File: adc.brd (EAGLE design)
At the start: 87.6 x 89.9 mm, 77 parts, among them IC13 4051D, IC5 4051D, IC6 4051D, U1 ADV7173KSTZ, U2 AD5308ARUZ, U3 AD7927BRUZ, U4 ADV7173KSTZ, U5 AD5308ARUZ, U6 AD5308ARUZ, U7 AD5308ARUZ

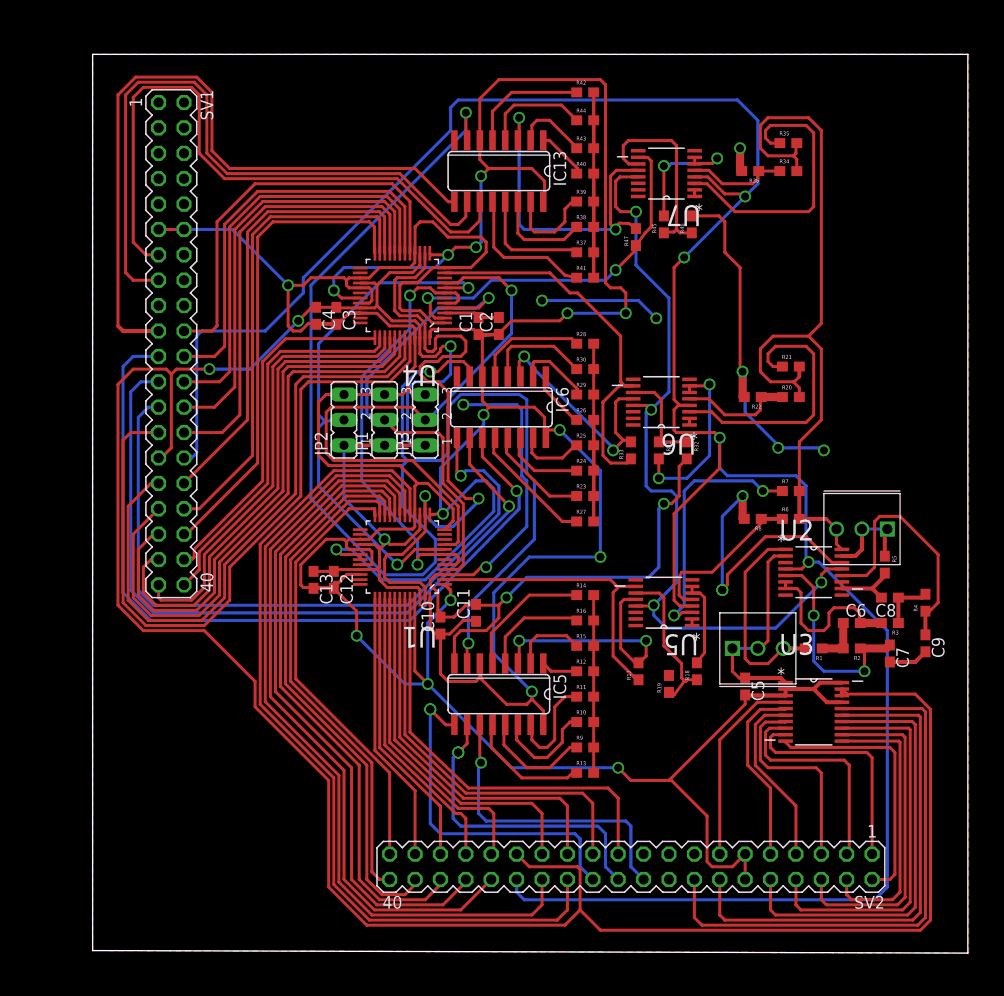
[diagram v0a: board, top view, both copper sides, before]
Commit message: autalização
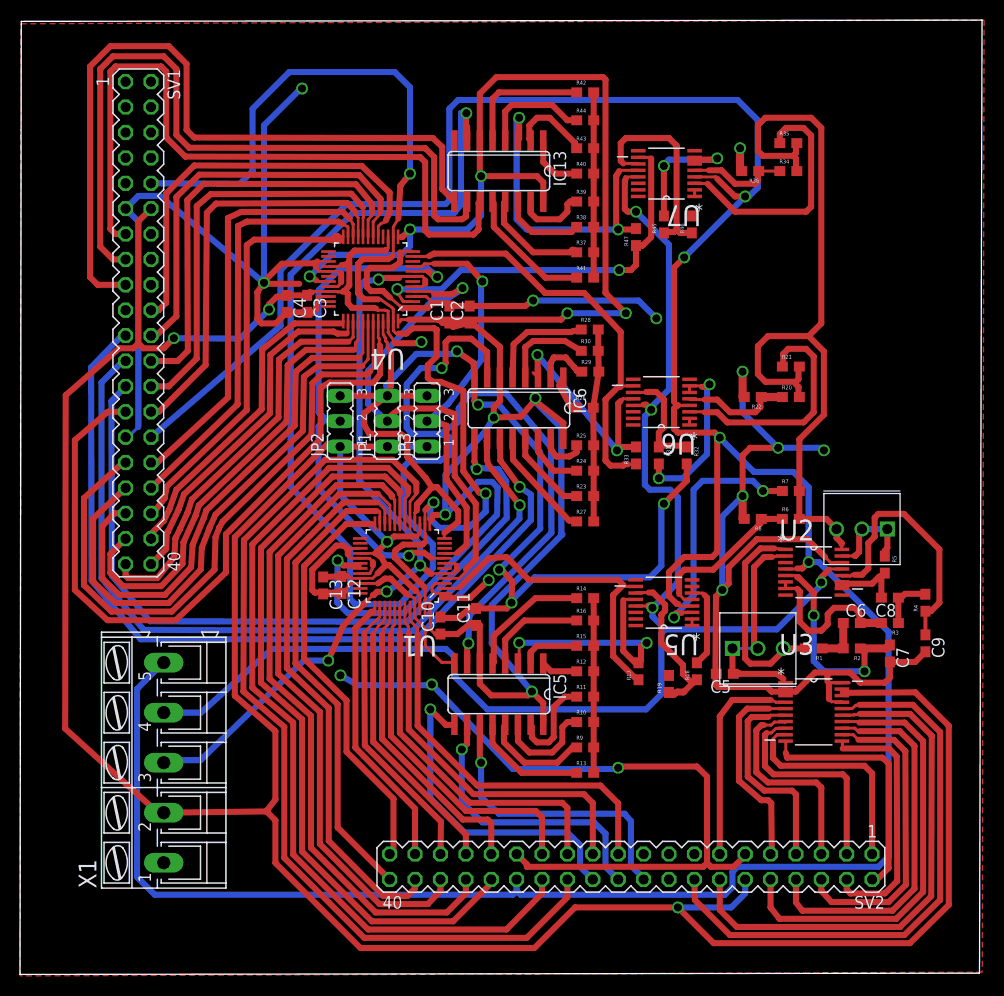
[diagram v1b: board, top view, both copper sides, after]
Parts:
- added X1: (no value), con-ptr500:AK300/5
- moved SV1 3.90 mm to (1.27, 56.9)
- moved U4 3.58 mm to (24.5, 61.3)
- moved C3 3.16 mm to (18.2, 58.9)
- moved C4 3.16 mm to (16.1, 58.9)
- moved C1 3.14 mm to (32.4, 57.8)
- moved C2 3.14 mm to (34.4, 57.8)
- moved C5 2.40 mm to (59.9, 21.8), turned to 180 degrees
- moved R29 2.34 mm to (46.5, 52.1)
- moved R30 1.89 mm to (46.4, 54.2)
- moved IC6 1.76 mm to (39.3, 48.4)
- moved R28 1.49 mm to (46.4, 56.3)
- moved R26 1.22 mm to (45.9, 48.5)
- moved C13 1.12 mm to (19.8, 30.7)
- moved C12 0.92 mm to (21.6, 30.7)
- moved U1 0.89 mm to (27.7, 32.6)
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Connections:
- removed net DGND: C12.2, C13.2, C3.2, C4.2, C5.2, JP1.3, JP2.3, JP3.3, SV1.11, SV1.12, SV2.11, SV2.12, U1.1, U1.12, U1.16, U1.27, U1.29, U1.32, U1.34, U1.45, U3.17, U3.2, U3.20, U3.3, U4.1, U4.12, U4.16, U4.27, U4.29, U4.32, U4.34, U4.45
- net +2,5V_ADCREF: now also X1.3
- net +5V: now also X1.5
- net -5V: now also X1.4
- net DCLK: now also SV1.10
- net GND: now also C12.2, C13.2, C3.2, C4.2, C5.2, JP1.3, JP2.3, JP3.3, SV1.11, SV1.29, SV2.11, SV2.29, U1.1, U1.12, U1.16, U1.27, U1.29, U1.32, U1.34, U1.45, U3.17, U3.2, U3.20, U3.3, U4.1, U4.12, U4.27, U4.29, U4.32, U4.34, U4.45, X1.1
- net N$93: now also SV1.17; no longer SV1.19
- net VDD: now also SV1.12, SV2.12, X1.2; no longer SV1.29, SV2.29
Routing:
- net GND: track 169.2 -> 475.0 mm, vias 12 -> 19
- net DGND: track 275.2 -> 0.00 mm, vias 5 -> 0
- net -5V: track 79.5 -> 142.3 mm
- net +5V: track 248.5 -> 309.9 mm
- net DCLK: track 68.3 -> 115.1 mm, vias 2 -> 3
- net VDD: track 295.7 -> 335.1 mm
- net +2,5V_ADCREF: track 45.6 -> 79.7 mm, vias 2 -> 4
- net N$102: track 45.2 -> 18.5 mm
- net VEE: track 139.6 -> 161.6 mm
- net S2: track 59.2 -> 41.2 mm
- net N$48: track 35.6 -> 19.2 mm
- net N$95: track 64.4 -> 72.4 mm
- net N$23: track 86.8 -> 94.6 mm
- net N$98: track 80.7 -> 87.4 mm
- net N$94: track 67.1 -> 73.6 mm
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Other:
- board size 87.6 x 89.9 mm -> 96.2 x 95.5 mm
